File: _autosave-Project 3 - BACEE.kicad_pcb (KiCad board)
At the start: 4 copper layers, 40.4 x 29.7 mm, 17 parts, among them J1 Digital pins, J2 Serial, J3 ICSP, J4 I2C, U1 DS1337S, U2 24LC1025, U3 24LC1025, U4 ATMEGA328P-AU, Y1 Crystal 32 MHz, Y2 Crystal 16 MHz

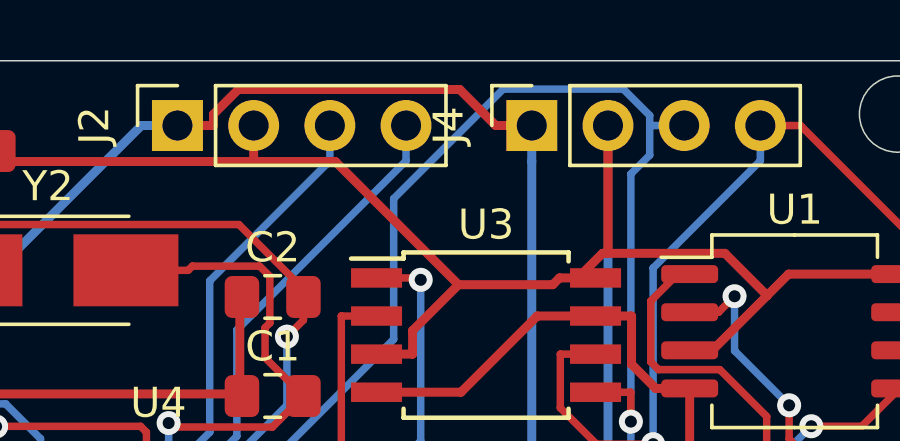
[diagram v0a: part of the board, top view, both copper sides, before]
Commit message: Added the gerber files.
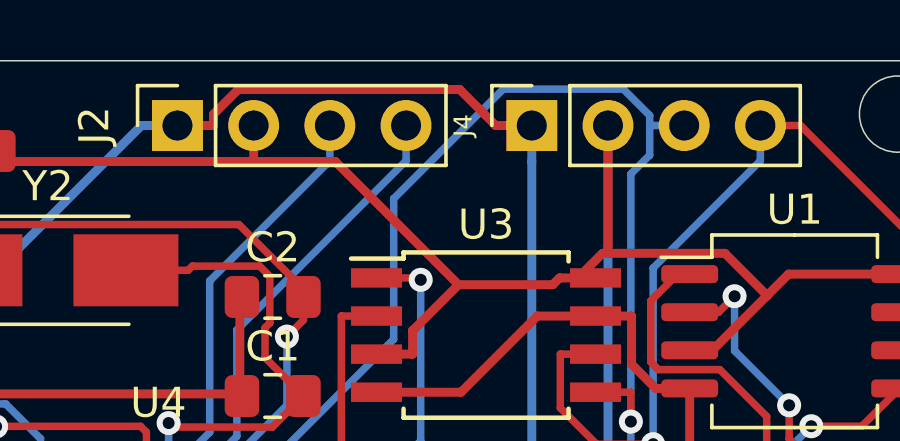
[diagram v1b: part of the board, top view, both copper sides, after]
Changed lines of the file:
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@@
     (pcbplotparams
       (layerselection 0x010fc_ffffffff)
-      (usegerberextensions false)
+      (usegerberextensions true)
       (usegerberattributes true)
       (usegerberadvancedattributes true)
@@
       (outputformat 1)
       (mirror false)
-      (drillshape 1)
+      (drillshape 0)
       (scaleselection 1)
-      (outputdirectory ""))
+      (outputdirectory "BACEE-Gerbers/"))
   )
   (net 0 "")
@@
     (descr "Through hole straight socket strip, 1x04, 2.54mm pitch, single row (from Kicad 4.0.7), script generated")
     (tags "Through hole socket strip THT 1x04 2.54mm single row")
-    (fp_text reference J4 (at 0 -2.77 90) (layer F.SilkS)
-      (effects (font (size 1 1) (thickness 0.15)))
+    (fp_text reference J4 (at 0 -2.286 90) (layer F.SilkS)
+      (effects (font (size 0.6 0.6) (thickness 0.15)))
     )
     (fp_text value I2C (at 0 10.39 90) (layer F.Fab)
